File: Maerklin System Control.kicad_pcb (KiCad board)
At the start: 2 copper layers, 83.8 x 73 mm, 16 parts, among them J1 Female Header, J2 Input, J3 Output, J4 Female Header Left, J5 Female Header Right, Q1 IRF3205, SW1 UP, SW2 RIGHT, SW3 DOWN, SW4 LEFT, SW5 SELECT, SW6 BACK

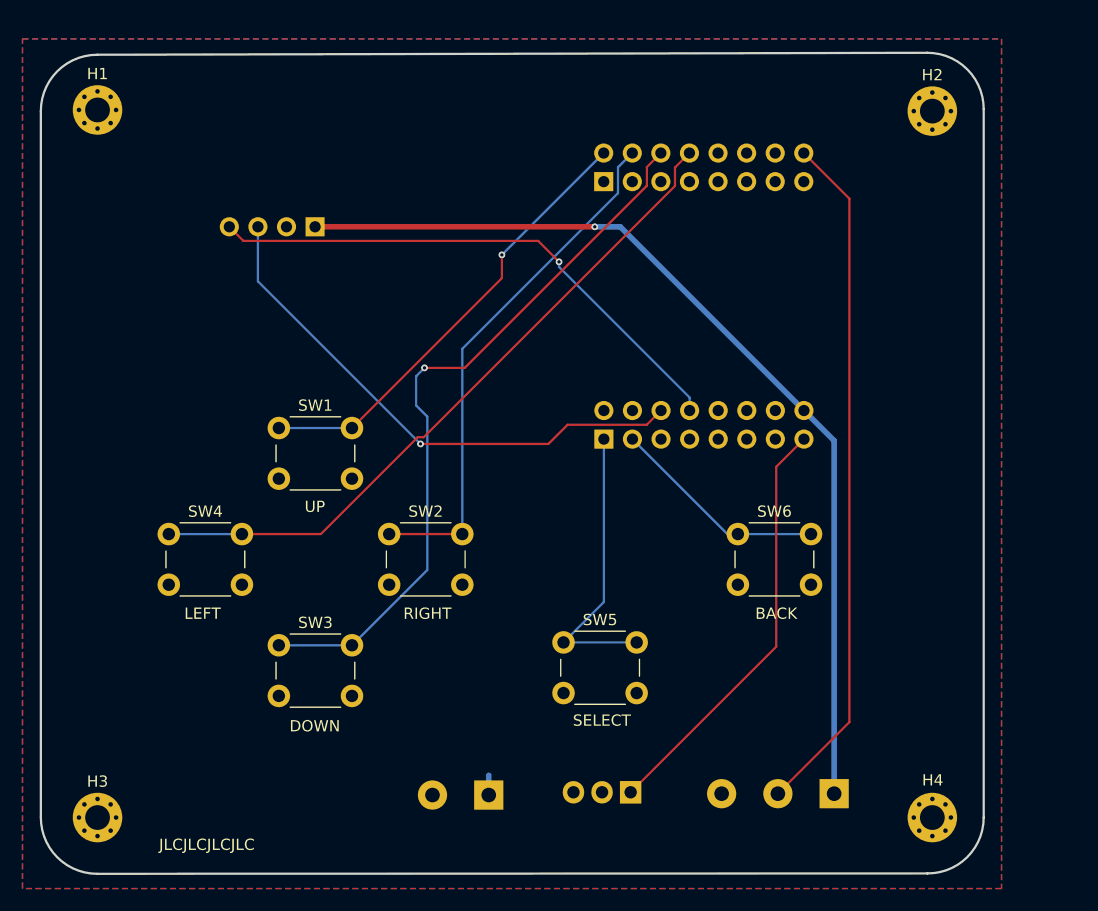
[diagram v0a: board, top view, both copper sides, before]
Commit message: latest v1.1 iteration
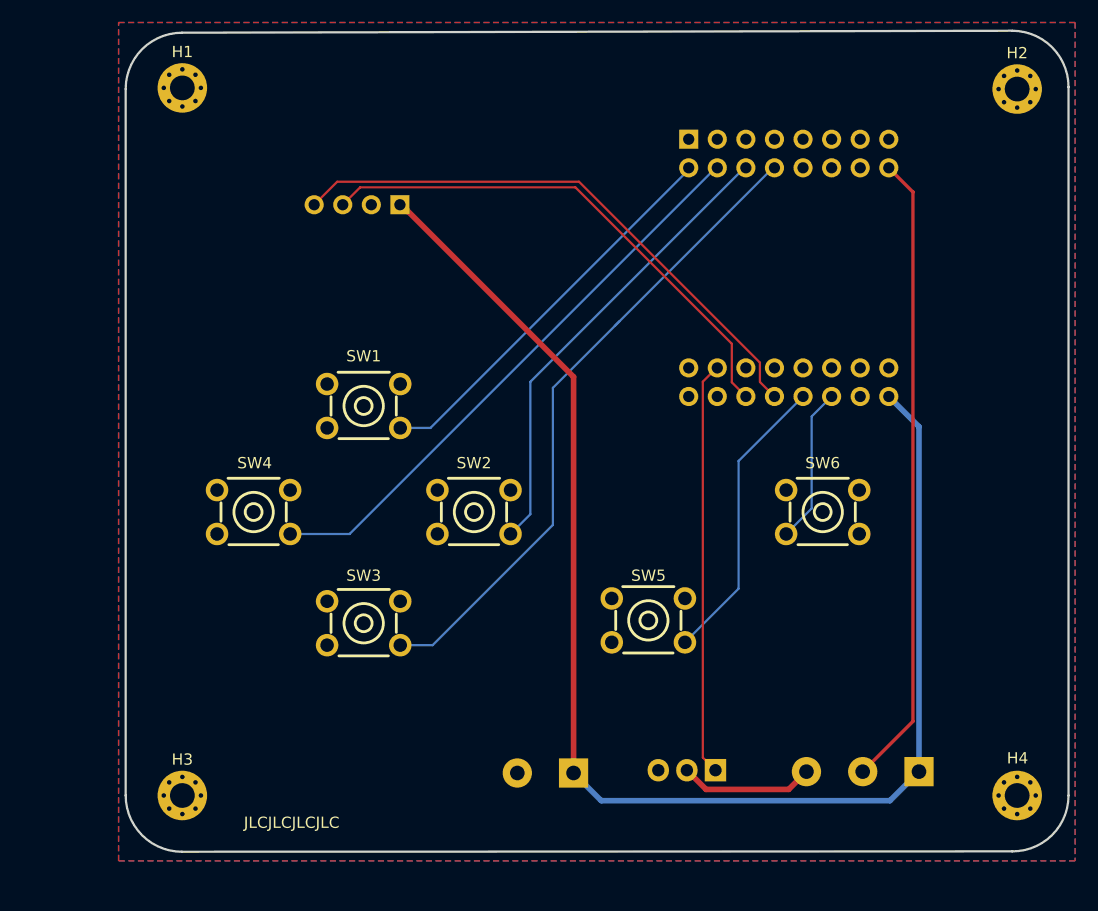
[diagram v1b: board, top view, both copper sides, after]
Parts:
- removed J5: Female Header Right, Connector_PinSocket_2.54mm:PinSocket_2x08_P2.54mm_Vertical
- J4: value Female Header Left -> Conn_S3 Mini; footprint Connector_PinSocket_2.54mm:PinSocket_2x08_P2.54mm_Vertical -> wemos:PinSocket_S3 Mini
- SW1, SW2, SW3, SW4, SW5, SW6: footprint Button_Switch_THT:SW_PUSH_6mm_H4.3mm -> easyeda2kicad:KEY-TH_4P-L6.0-W6.0-P3.90-LS7.8
- moved J4 18.3 mm to (120.5, 44.1)
- moved J3 7.79 mm to (132.1, 88.6)
- moved H1 7.79 mm to (66.6, 27.8)
- moved H3 7.79 mm to (66.6, 90.7)
- moved J1 7.79 mm to (85.9, 38.2)
- moved J2 7.79 mm to (101.4, 88.7)
- moved Q1 7.79 mm to (114.0, 88.4)
- moved SW1 7.79 mm to (82.7, 56.1)
- moved SW2 7.79 mm to (92.5, 65.5)
- moved SW3 7.79 mm to (82.7, 75.4)
- moved SW4 7.79 mm to (72.9, 65.5)
- moved SW5 7.79 mm to (108.0, 75.1)
- moved SW6 7.79 mm to (123.5, 65.5)
- moved H2 7.79 mm to (140.8, 27.9)
- moved H4 7.79 mm to (140.8, 90.7)
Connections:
- net DIN renamed DOUT
- J3 pad 3: GND -> GND1
- J4 pad 10: unconnected-(J4-GPIO7-Pad10) -> LEFT
- J4 pad 11: unconnected-(J4-GPIO11-Pad11) -> RIGHT
- J4 pad 12: unconnected-(J4-GPIO8-Pad12) -> DOWN
- J4 pad 2: UP -> unconnected-(J4-IO2-Pad2)
- J4 pad 4: RIGHT -> unconnected-(J4-IO12-Pad4)
- J4 pad 6: DOWN -> unconnected-(J4-IO11-Pad6)
- J4 pad 8: LEFT -> unconnected-(J4-+3V3-Pad8)
- J4 pad 9: unconnected-(J4-GPIO13-Pad9) -> UP
- Q1 pad 2: GND -> GND1
- SW1 pad 2: GND -> UP
- SW2 pad 2: GND -> RIGHT
- SW3 pad 2: GND -> DOWN
- SW4 pad 2: GND -> LEFT
- SW5 pad 2: GND -> SELECT
- SW6 pad 2: GND -> BACK
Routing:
- net +5V: track 87.3 -> 124.2 mm, vias 1 -> 0
- net GND1: track 0.00 -> 12.0 mm
- net LEFT: track 61.3 -> 51.4 mm
- net DOWN: track 64.5 -> 58.5 mm, vias 1 -> 0
- net BACK: track 19.4 -> 13.9 mm
- net RIGHT: track 46.6 -> 41.3 mm
- net UP: track 40.2 -> 35.3 mm, vias 1 -> 0
- net DOUT: track 61.2 -> 56.5 mm
- net SDA: track 48.6 -> 50.7 mm, vias 1 -> 0
- net SCK: track 47.9 -> 46.2 mm, vias 1 -> 0
- net MOSFET: track 37.8 -> 36.8 mm
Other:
- board text added: "DOUT"
- board text removed: "DIN"
